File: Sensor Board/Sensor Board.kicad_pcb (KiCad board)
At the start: 2 copper layers, 40 x 40 mm, 34 parts, among them J1 Programming Header, J2 Irradience Sensor, J3 Micro_SD_Card, J4 CAN Bus Connector, U1 PIC18F26K83, U2 INA180, U4 MCP2562, U5 INA180, Y1 12MHz Crystal

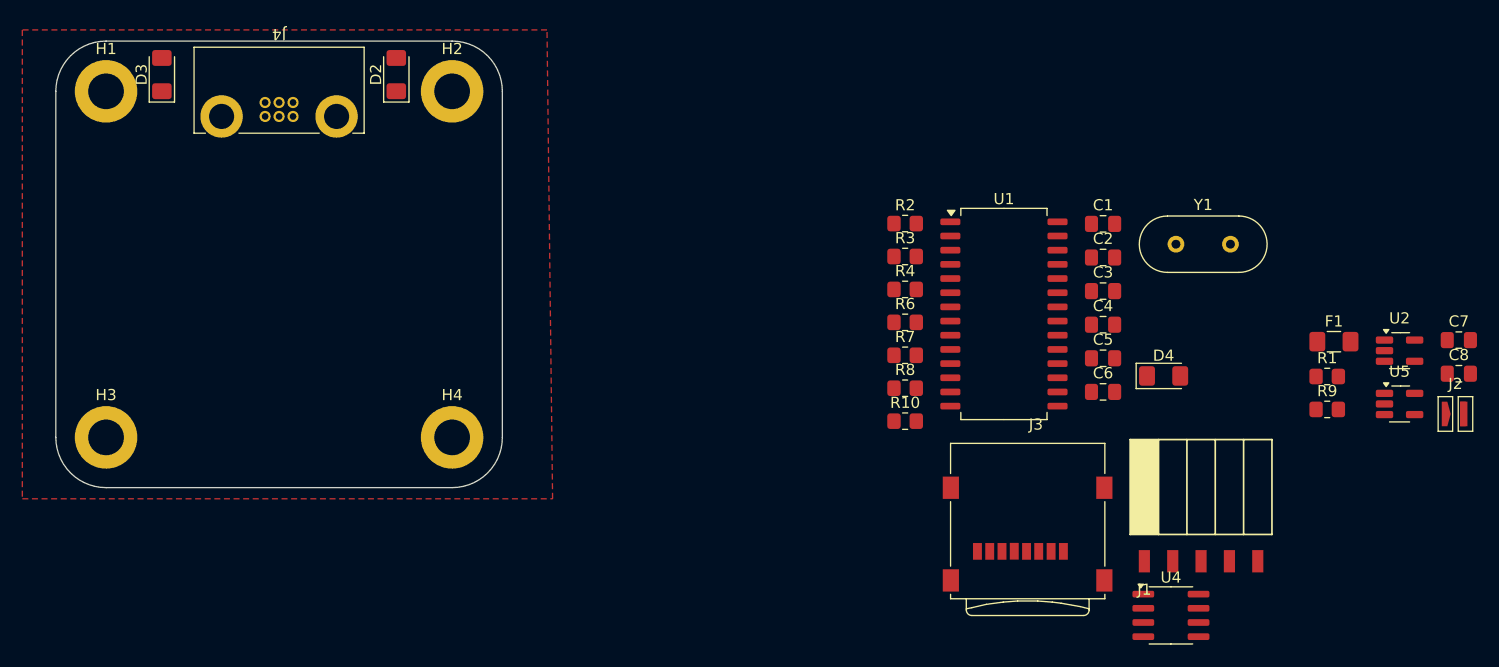
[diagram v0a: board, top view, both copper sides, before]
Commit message: Fix review items
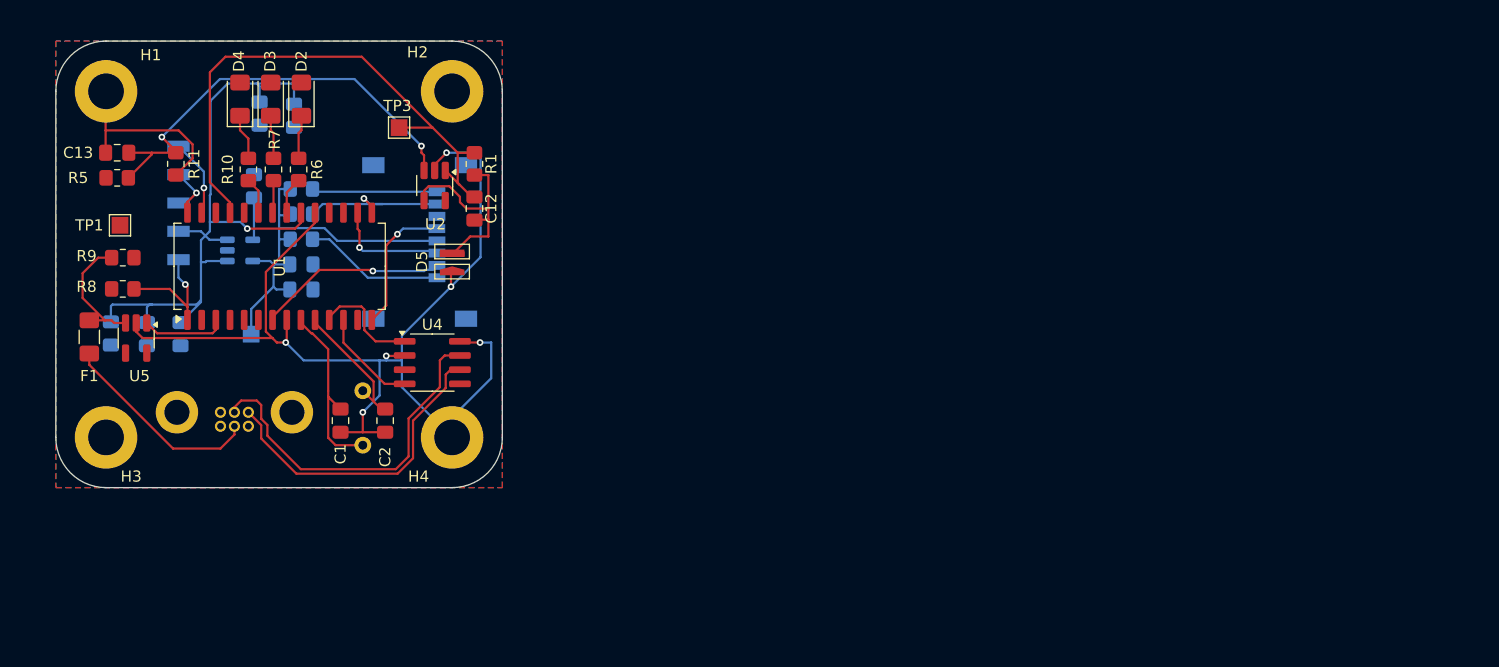
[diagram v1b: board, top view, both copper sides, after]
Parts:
- removed C8: 0.1uF, Capacitor_SMD:C_0805_2012Metric_Pad1.18x1.45mm_HandSolder
- removed J2: Irradience Sensor, Canhw:P16612-011CA
- added C10: 10nF, Capacitor_SMD:C_0805_2012Metric_Pad1.18x1.45mm_HandSolder, B.Cu at (117.8, 63.0)
- added C11: 1uF, Capacitor_SMD:C_0805_2012Metric_Pad1.18x1.45mm_HandSolder, B.Cu at (122.0, 72.2)
- added C12: 1.6pF, Capacitor_SMD:C_0805_2012Metric_Pad1.18x1.45mm_HandSolder, F.Cu at (137.5, 65.0)
- added C13: 1uF, Capacitor_SMD:C_0805_2012Metric_Pad1.18x1.45mm_HandSolder, F.Cu at (105.5, 60.0)
- added C9: 1uF, Capacitor_SMD:C_0805_2012Metric_Pad1.18x1.45mm_HandSolder, B.Cu at (104.9, 76.2)
- added D5: Irr Sense, Canhw:P16612-011CA, F.Cu at (135.5, 69.8)
- added R11: 1kR, Resistor_SMD:R_0805_2012Metric_Pad1.20x1.40mm_HandSolder, F.Cu at (110.8, 61.0)
- added R5: 47kR, Resistor_SMD:R_0805_2012Metric_Pad1.20x1.40mm_HandSolder, F.Cu at (105.5, 62.2)
- added TP1: 5v, TestPoint:TestPoint_Pad_1.5x1.5mm, F.Cu at (105.8, 66.5)
- added TP2: 3.3v, TestPoint:TestPoint_Pad_1.5x1.5mm, B.Cu at (117.5, 76.2)
- added TP3: TestPoint, TestPoint:TestPoint_Pad_1.5x1.5mm, F.Cu at (130.8, 57.8)
- added U3: SPX3819M5-L-3-3, Package_TO_SOT_SMD:SOT-23-5, B.Cu at (116.5, 68.8)
- C3, C4, C5, C6, C7, J1, J3, J4, R2, R3, R4, Y1: moved to B.Cu
- R1: value 180kR -> 5MR
- R10, R6, R7: value 330R -> 150R
- moved U5 113.3 mm to (107.2, 76.6), turned to -90 degrees
- moved F1 111.5 mm to (103.0, 76.5), turned to 90 degrees
- moved C7 109.3 mm to (118.2, 56.5), turned to -90 degrees
- moved R9 108.7 mm to (106.0, 69.4), turned to 180 degrees
- moved J1 94.2 mm to (111.0, 59.4), turned to -90 degrees
- moved U2 87.7 mm to (133.9, 62.9), turned to -90 degrees
- moved D4 86.4 mm to (116.5, 55.2), turned to 90 degrees
- moved C6 85.8 mm to (108.2, 76.2), turned to 90 degrees
- moved C5 82.7 mm to (111.2, 76.2), turned to 90 degrees
- moved R1 78.7 mm to (137.5, 61.0), turned to 90 degrees
- moved Y1 75.0 mm to (127.5, 86.2), turned to 90 degrees
- moved C4 74.9 mm to (121.3, 56.7), turned to -90 degrees
- moved C3 71.8 mm to (122.0, 70.0), turned to 180 degrees
- moved R8 70.6 mm to (106.0, 72.2)
- moved C1 70.5 mm to (125.5, 84.0), turned to -90 degrees
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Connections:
- net CURR_SENSE renamed /CURR_SENSE
- C1 pad 2: Net-(C1-Pad2) -> GND
- C2 pad 2: Net-(C1-Pad2) -> GND
- C3 pad 2: +5V -> +3.3V
- J3 pad 4: +5V -> +3.3V
- J3 pad 9: unconnected-(J3-SHIELD-Pad9) -> GND
- J4 pad 2: CANL -> /CANH
- J4 pad 3: CANH -> /CANL
- R1 pad 1: +5V -> Net-(D5-A)
- R1 pad 2: Net-(U2-IN-) -> /IRR_SENSE
- R2 pad 1: +5V -> +3.3V
- R3 pad 1: +5V -> +3.3V
- R4 pad 1: +5V -> +3.3V
- U1 pad 25: IRR_SENSE -> /IRR_SENSE
- U2 pad 1: IRR_SENSE -> /IRR_SENSE
- U2 pad 3: +5V -> Net-(U2-IN+)
- U2 pad 4: Net-(U2-IN-) -> Net-(D5-A)
- U4 pad 1: /CANRX -> /CANTX
- U4 pad 4: /CANTX -> /CANRX
- U4 pad 6: CANL -> /CANL
- U4 pad 7: CANH -> /CANH
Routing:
- net GND: track 0.00 -> 120.8 mm, vias 0 -> 6
- net +5V: track 0.00 -> 61.2 mm, vias 0 -> 1
- net /IRR_SENSE: track 0.00 -> 50.7 mm
- net Net-(U2-IN+): track 0.00 -> 39.4 mm, vias 0 -> 2
- net +3.3V: track 0.00 -> 36.8 mm
- net /CANH: track 0.00 -> 32.4 mm
- net /CANL: track 0.00 -> 28.5 mm
- net Net-(D5-A): track 0.00 -> 20.0 mm
- net Net-(J4-Pin_5): track 0.00 -> 18.4 mm
- net /PIC_MICRO_SD_CS: track 0.00 -> 17.0 mm, vias 0 -> 1
- net /OSC1: track 0.00 -> 16.6 mm
- net /PIC_MICRO_SD_SDI: track 0.00 -> 14.9 mm, vias 0 -> 1
- net Net-(J3-DAT2): track 0.00 -> 12.6 mm
- net /PIC_MICRO_SD_SCK: track 0.00 -> 12.4 mm, vias 0 -> 1
- net /OSC2: track 0.00 -> 12.2 mm
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- added copper zone on B.Cu, net GND
